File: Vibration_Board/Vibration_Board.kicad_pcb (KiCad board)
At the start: 4 copper layers, 53 parts, among them J1 Debugging Connector, J2 Micro_SD_Card, J3 Gecko Connector, J4 Gecko Connector, J5 G125-MH104M4-04AD000P, J6 Gecko Connector, J7 Gecko Connector, U1 SHT31-DIS-B2.5KS, U10 MCP2562, U2 INA180A1, U3 SPX3819M5-L-3-3, U4 STM32H745ZIT6, Y1 24MHz crystal

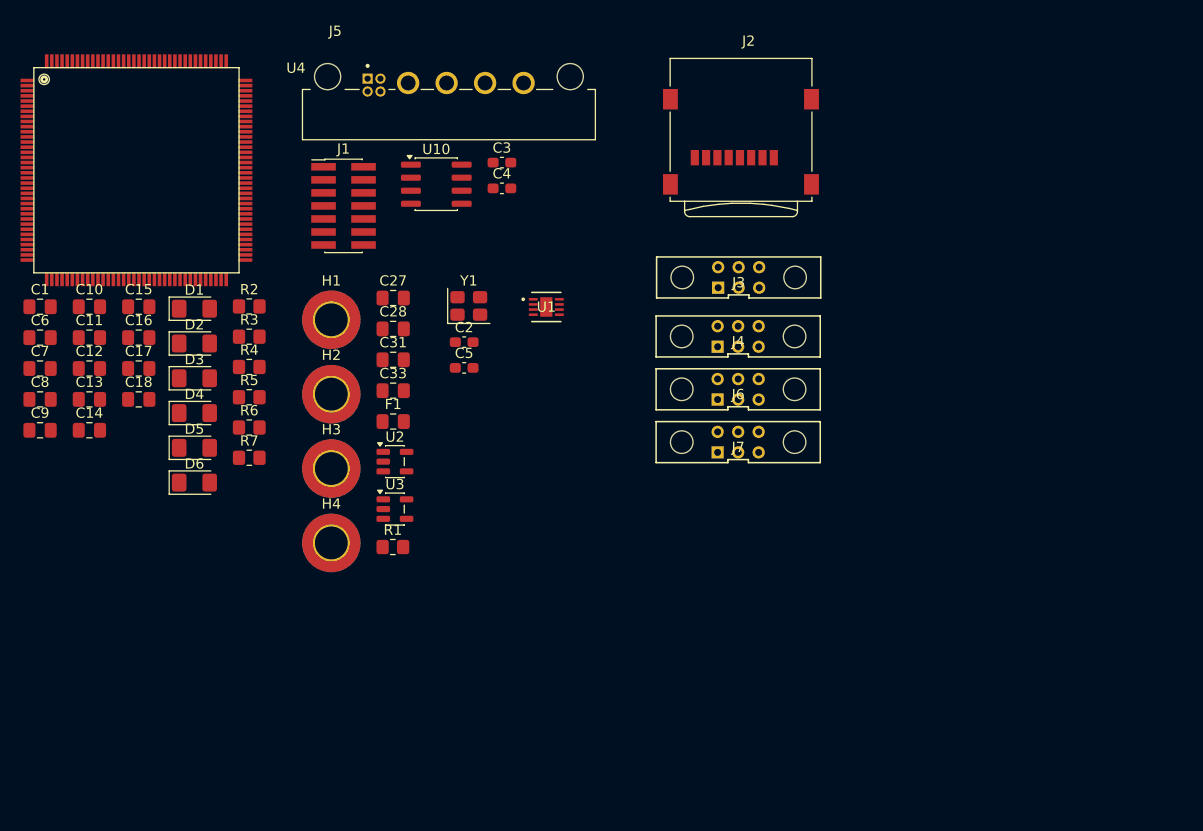
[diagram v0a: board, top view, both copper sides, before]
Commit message: everything added
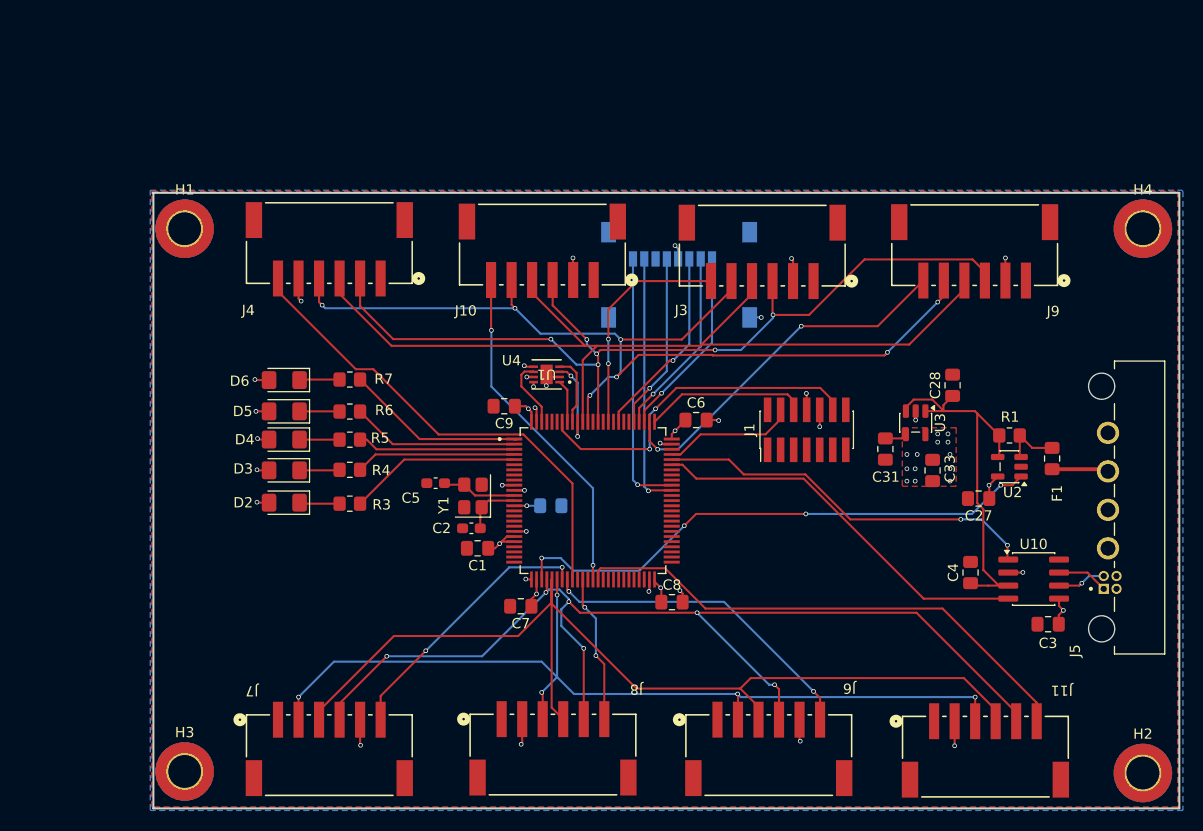
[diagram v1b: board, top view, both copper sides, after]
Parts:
- removed C11, C12, C13, C14, C15, C16, C17, C18: 1uF, Capacitor_SMD:C_0805_2012Metric_Pad1.18x1.45mm_HandSolder
- removed D1: LED, LED_SMD:LED_1206_3216Metric_Pad1.42x1.75mm_HandSolder
- removed R2: R_US, Resistor_SMD:R_0805_2012Metric_Pad1.20x1.40mm_HandSolder
- added J10: Conn_01x06_Pin, jst:CONN6_S6B-PH_JST, F.Cu at (50.9, 18.5)
- added J11: Conn_01x06_Pin, jst:CONN6_S6B-PH_JST, F.Cu at (94.0, 68.5)
- added J8: Conn_01x06_Pin, jst:CONN6_S6B-PH_JST, F.Cu at (51.9, 68.3)
- added J9: Conn_01x06_Pin, jst:CONN6_S6B-PH_JST, F.Cu at (93.0, 18.6)
- C10, J2: moved to B.Cu
- C3, C4: footprint Capacitor_SMD:C_0603_1608Metric_Pad1.08x0.95mm_HandSolder -> Capacitor_SMD:C_0805_2012Metric_Pad1.18x1.45mm_HandSolder
- J3, J4, J6, J7: value Gecko Connector -> Conn_01x06_Pin; footprint G125-MH104M4-04AD000P:connector_Harwin_M80-5000642 -> jst:CONN6_S6B-PH_JST
- U4: value STM32H745ZIT6 -> STM32H750VBT6TR; footprint STM32H745ZIT6:LQFP144 -> STM32H745ZIT6:QFP50P1600X1600X160-100N
- moved H2 87.3 mm to (109.4, 70.0)
- moved H4 84.8 mm to (109.4, 17.0)
- moved J5 77.5 mm to (109.1, 44.2), turned to 90 degrees
- moved U10 69.8 mm to (98.8, 51.1)
- moved C3 69.7 mm to (100.2, 55.5)
- moved C8 64.7 mm to (63.5, 53.4)
- moved C6 64.4 mm to (65.8, 35.6)
- moved F1 64.3 mm to (100.5, 39.4), turned to 90 degrees
- moved R1 61.1 mm to (96.4, 37.1), turned to 180 degrees
- moved C27 60.3 mm to (93.4, 43.3), turned to 180 degrees
- moved U2 59.9 mm to (96.4, 40.2), turned to 180 degrees
- moved C4 59.1 mm to (92.6, 50.5), turned to 90 degrees
- moved C28 54.8 mm to (90.8, 32.3), turned to 90 degrees
- moved U4 54.8 mm to (55.8, 43.5)
- moved C33 53.1 mm to (88.9, 40.6), turned to -90 degrees
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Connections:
- C10 pad 1: +3.3VD -> Net-(U4A-~{RST})
- J3 pad 1: unconnected-(J3-Pin_1-Pad1) -> GND
- J3 pad 2: unconnected-(J3-Pin_2-Pad2) -> +3.3VD
- J3 pad 3: unconnected-(J3-Pin_3-Pad3) -> /Connectors/MOSI_2
- J3 pad 4: unconnected-(J3-Pin_4-Pad4) -> /Connectors/MISO_2
- J3 pad 5: unconnected-(J3-Pin_5-Pad5) -> /Connectors/SCK_2
- J3 pad 6: unconnected-(J3-Pin_6-Pad6) -> /ACCEL_CS4
- J4 pad 1: unconnected-(J4-Pin_1-Pad1) -> GND
- J4 pad 2: unconnected-(J4-Pin_2-Pad2) -> /Connectors/MOSI_2
- J4 pad 3: unconnected-(J4-Pin_3-Pad3) -> /Connectors/MISO_2
- J4 pad 4: unconnected-(J4-Pin_4-Pad4) -> /Connectors/SCK_2
- J4 pad 5: unconnected-(J4-Pin_5-Pad5) -> +3.3VD
- J4 pad 6: unconnected-(J4-Pin_6-Pad6) -> /ACCEL_CS3
- J6 pad 1: unconnected-(J6-Pin_1-Pad1) -> GND
- J6 pad 2: unconnected-(J6-Pin_2-Pad2) -> /MOSI
- J6 pad 3: unconnected-(J6-Pin_3-Pad3) -> /MISO
- J6 pad 4: unconnected-(J6-Pin_4-Pad4) -> /SCK
- J6 pad 5: unconnected-(J6-Pin_5-Pad5) -> +3.3VD
- J6 pad 6: unconnected-(J6-Pin_6-Pad6) -> /ACCEL_CS2
- J7 pad 1: unconnected-(J7-Pin_1-Pad1) -> GND
- J7 pad 2: unconnected-(J7-Pin_2-Pad2) -> /MOSI
- J7 pad 3: unconnected-(J7-Pin_3-Pad3) -> /MISO
- J7 pad 4: unconnected-(J7-Pin_4-Pad4) -> /SCK
- J7 pad 5: unconnected-(J7-Pin_5-Pad5) -> +3.3VD
- J7 pad 6: unconnected-(J7-Pin_6-Pad6) -> /ACCEL_CS1
- U1 pad 6: /SENSORS/TEMP_RESET -> /SENSOR_RESET
- U4 pad 10: unconnected-(U4-PC14/OSC32_IN-Pad10) -> GND
- U4 pad 100: /RX -> +3.3VD
- U4 pad 11: unconnected-(U4-PC15/OSC32_OUT-Pad11) -> +3.3VD
- U4 pad 12: GND -> /MCU/MCLK_IN
- U4 pad 13: +3.3VD -> /MCU/MCLK_OUT
- U4 pad 14: unconnected-(U4-VSSSMPS-Pad14) -> Net-(U4A-~{RST})
- U4 pad 18: GND -> unconnected-(U4C-PC3_C/ADC3_INP1-Pad18)
- U4 pad 19: +3.3VD -> GND
- U4 pad 20: unconnected-(U4-PF6-Pad20) -> +3.3VD
- U4 pad 21: unconnected-(U4-PF7-Pad21) -> +3.3VD
- U4 pad 25: /MCU/MCLK_OUT -> unconnected-(U4A-PA3/TIM2_CH4/TIM5_CH4/LPTIM5_OUT/TIM15_CH2/USART2_RX/LCD_B2/OTG_HS_ULPI_D0/ETH_MII_COL/LCD_B5/EVENTOUT/ADC12_INP15-Pad25)
- U4 pad 26: /MCU/MCLK_IN -> GND
- U4 pad 27: /MCLR -> +3.3VD
- U4 pad 28: unconnected-(U4-PC0-Pad28) -> /CUR_SEN
- U4 pad 29: unconnected-(U4-PC1-Pad29) -> /SCK
- U4 pad 30: unconnected-(U4-PC2_C-Pad30) -> /MISO
- U4 pad 31: unconnected-(U4-PC3_C-Pad31) -> /MOSI
- U4 pad 32: +3.3VD -> /ACCEL_CS1
- U4 pad 33: GND -> /ACCEL_CS2
- U4 pad 34: GND -> /ACCEL_CS3
- U4 pad 35: GND -> unconnected-(U4B-PB1/TIM1_CH3N/TIM3_CH4/TIM8_CH3N/DFSDM_DATIN1/LCD_R6/OTG_HS_ULPI_D2/ETH_MII_RXD3/LCD_G0/EVENTOUT/ADC12_INP5/COMP_1_INM-Pad35)
- U4 pad 36: +3.3VD -> /ACCEL_CS5
- U4 pad 38: unconnected-(U4-PA1-Pad38) -> /ACCEL_CS7
- U4 pad 39: unconnected-(U4-PA2-Pad39) -> /ACCEL_CS8
- U4 pad 41: GND -> unconnected-(U4E-PE11/TIM1_CH2/DFSDM_CKIN4/SPI4_NSS/SAI2_SD_B/FMC_D8/FMC_DA8/LCD_G3/EVENTOUT/COMP_2_INP-Pad41)
- U4 pad 42: +3.3VD -> unconnected-(U4E-PE12/TIM1_CH3N/DFSDM_DATIN5/SPI4_SCK/SAI2_SCK_B/FMC_D9/FMC_DA9/COMP_1_OUT/LCD_B4/EVENTOUT-Pad42)
- U4 pad 43: /SCK -> unconnected-(U4E-PE13/TIM1_CH3/DFSDM_CKIN5/SPI4_MISO/SAI2_FS_B/FMC_D10/FMC_DA10/COMP_2_OUT/LCD_DE/EVENTOUT-Pad43)
- U4 pad 44: /MISO -> unconnected-(U4E-PE14/TIM1_CH4/SPI4_MOSI/SAI2_MCK_B/FMC_D11/FMC_DA11/LCD_CLK/EVENTOUT-Pad44)
- U4 pad 45: /MOSI -> unconnected-(U4E-PE15/TIM1_BKIN/HDMI__TIM1_BKIN/FMC_D12/FMC_DA12/TIM1_BKIN_COMP12/LCD_R7/EVENTOUT-Pad45)
- U4 pad 46: /ACCEL_CS1 -> unconnected-(U4B-PB10/TIM2_CH3/HRTIM_SCOUT/LPTIM2_IN1/I2C2_SCL/SPI2_SCK/I2S2_CK/DFSDM_DATIN7/USART3_TX/QUADSPI_BK1_NCS/OTG_HS_ULPI_D3/ETH_MII_RX_ER/LCD_G4/EVENTOUT-Pad46)
- U4 pad 47: /ACCEL_CS2 -> unconnected-(U4B-PB11/TIM2_CH4/HRTIM_SCIN/LPTIM2_ETR/I2C2_SDA/DFSDM_CKIN7/USART3_RX/OTG_HS_ULPI_D4/ETH_MII_TX_EN/ETH_RMII_TX_EN/LCD_G5/EVENTOUT-Pad47)
- U4 pad 48: /ACCEL_CS3 -> VCAP_1
- U4 pad 49: /ACCEL_CS4 -> GND
- U4 pad 50: unconnected-(U4-PB1-Pad50) -> +3.3VD
- U4 pad 55: GND -> unconnected-(U4D-PD8/DFSDM_CKIN3/SAI3_SCK_B/USART3_TX/SPDIFRX_IN1/FMC_D13/FMC_DA13/EVENTOUT-Pad55)
- U4 pad 56: +3.3VD -> unconnected-(U4D-PD9/DFSDM_DATIN3/SAI3_SD_B/USART3_RX/FDCAN2_RXFD_MODE/FMC_D14/FMC_DA14/EVENTOUT-Pad56)
- U4 pad 6: Net-(U4-VSS@1) -> unconnected-(U4A-VBAT-Pad6)
- U4 pad 65: unconnected-(U4-PE15-Pad65) -> /Connectors/DATA1
- U4 pad 66: unconnected-(U4-PB10-Pad66) -> /Connectors/DATA2
- U4 pad 69: GND -> unconnected-(U4A-PA10/TIM1_CH3/HRTIM_CHC2/LPUART1_RX/USART1_RX/FDCAN1_TXFD_MODE/OTG_FS_ID/MDIOS_MDIO/LCD_B4/DCMI_D1/LCD_B1/EVENTOUT-Pad69)
- U4 pad 7: +3.3VD -> unconnected-(U4C-PC13/EVENTOUT/RTC_TAMP_1/RTC_TS/WKUP2-Pad7)
- U4 pad 70: unconnected-(U4-VDDLDO@1-Pad70) -> /RX
- U4 pad 71: +3.3VD -> /TX
- U4 pad 72: unconnected-(U4-PB12-Pad72) -> /PGC
- U4 pad 73: unconnected-(U4-PB13-Pad73) -> VCAP
- U4 pad 74: unconnected-(U4-PB14-Pad74) -> GND
- U4 pad 75: unconnected-(U4-PB15-Pad75) -> +3.3VD
- U4 pad 76: unconnected-(U4-PD8-Pad76) -> /PGD
- U4 pad 77: unconnected-(U4-PD9-Pad77) -> /ACCEL_CS6
- U4 pad 78: unconnected-(U4-PD10-Pad78) -> /Connectors/DATA3
- U4 pad 79: +3.3VD -> /Connectors/DATA4
- U4 pad 80: GND -> /Connectors/SD_CLK
- U4 pad 83: unconnected-(U4-PD13-Pad83) -> /Connectors/SD_CS
- U4 pad 85: unconnected-(U4-PD15-Pad85) -> /ACCEL_CS4
- U4 pad 87: unconnected-(U4-PG7-Pad87) -> /Connectors/MOSI_2
- U4 pad 89: GND -> /Connectors/SCK_2
- U4 pad 90: unconnected-(U4-VDD50USB-Pad90) -> /Connectors/MISO_2
- U4 pad 91: unconnected-(U4-VDD33USB-Pad91) -> /I2C_ALERT
- U4 pad 92: +3.3VD -> /I2C_SCK
- U4 pad 93: unconnected-(U4-PC6-Pad93) -> /I2C_DATA
- U4 pad 94: unconnected-(U4-PC7-Pad94) -> /MCLR
- U4 pad 95: /Connectors/DATA1 -> unconnected-(U4B-PB8/TIM16_CH1/TIM4_CH3/DFSDM_CKIN7/I2C1_SCL/I2C4_SCL/SDMMC1_CKIN/UART4_RX/FDCAN1_RX/SDMMC2_D4/ETH_MII_TXD3/SDMMC1_D4/DCMI_D6/LCD_B6/EVENTOUT-Pad95)
- U4 pad 96: /Connectors/DATA2 -> unconnected-(U4B-PB9/TIM17_CH1/TIM4_CH4/DFSDM_DATIN7/I2C1_SDA/SPI2_NSS/I2S2_WS/I2C4_SDA/SDMMC1_CDIR/UART4_TX/FDCAN1_TX/SDMMC2_D5/I2C4_SMBA/SDMMC1_D5/DCMI_D7/LCD_B7/EVENTOUT-Pad96)
- U4 pad 98: unconnected-(U4-PA9-Pad98) -> /SENSOR_RESET
- U4 pad 99: unconnected-(U4-PA10-Pad99) -> GND
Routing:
- net /SCK: track 0.00 -> 106.1 mm, vias 0 -> 6
- net /MISO: track 0.00 -> 97.6 mm
- net /Connectors/SCK_2: track 0.00 -> 96.3 mm, vias 0 -> 7
- net /Connectors/MISO_2: track 0.00 -> 92.6 mm
- net /Connectors/MOSI_2: track 0.00 -> 90.4 mm, vias 0 -> 6
- net /MOSI: track 0.00 -> 90.2 mm, vias 0 -> 5
- net /CUR_SEN: track 0.00 -> 53.1 mm, vias 0 -> 4
- net /ACCEL_CS8: track 0.00 -> 50.9 mm
- net +3.3VD: track 0.00 -> 50.1 mm, vias 0 -> 37
- net /ACCEL_CS3: track 0.00 -> 47.1 mm
- net +5V: track 0.00 -> 39.3 mm
- net /RX: track 0.00 -> 38.2 mm
- net /TX: track 0.00 -> 37.6 mm, vias 0 -> 2
- net /ACCEL_CS6: track 0.00 -> 35.7 mm, vias 0 -> 2
- net /MCLR: track 0.00 -> 33.8 mm, vias 0 -> 2
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- added copper zone on F.Cu, net +3.3VD
- added copper zone on In1.Cu, net +3.3VD
- added copper zone on B.Cu, net GND
- added copper zone on F.Cu, net GND
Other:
- board outline added: 100 x 60 mm
